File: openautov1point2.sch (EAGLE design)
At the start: 78 parts, among them CN1 6p-2.54, CN2 6p-2.54, CN3 6p-2.54, IC1 NC7SZ14M5X, IC2 TJA1049, IC3 NCP1117CORRECT, J3 4p-2.54, Q1 s9013, Q2 s9013, U3 MMA7660FCR1, U5 A2235-H, U8 PCF85063TP, X3 BU-SMA-H, X4 ABS07-32.768KHZ

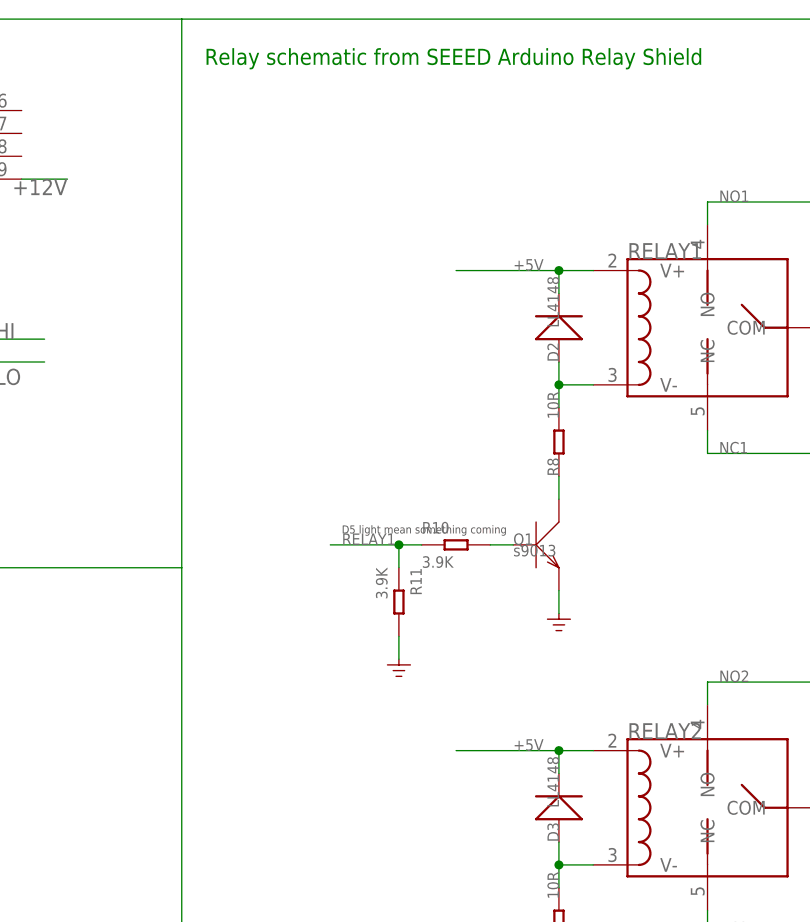
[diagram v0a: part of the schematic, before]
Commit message: updated after design review
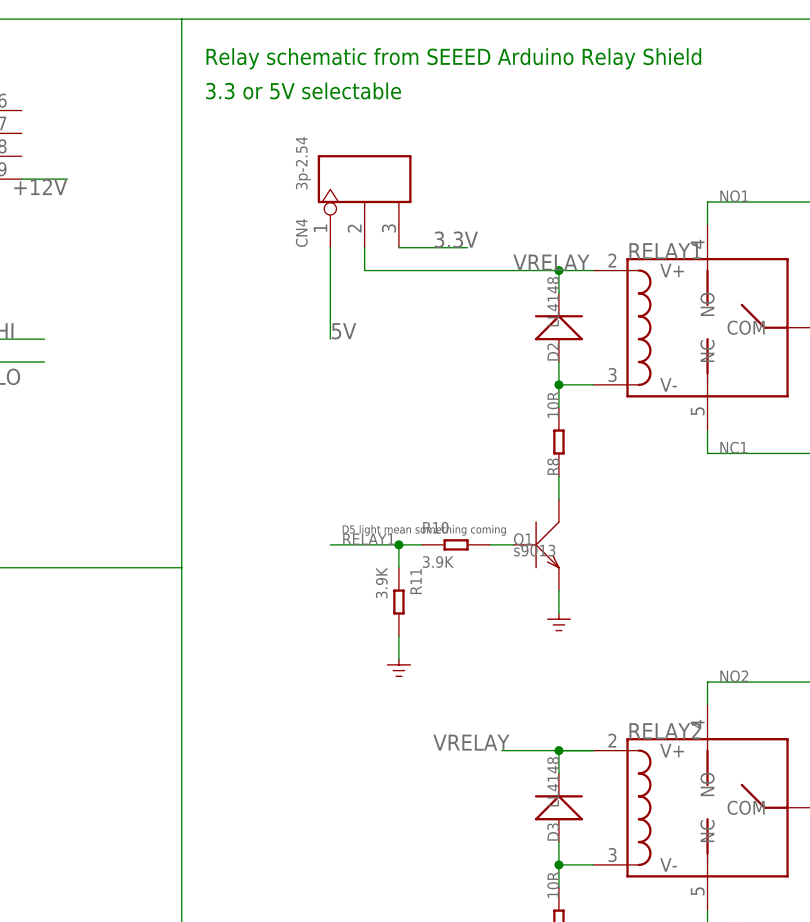
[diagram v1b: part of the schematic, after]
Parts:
- added CN4: 3p-2.54, Seeed-Connector:DIP-BLACK-MALE-HEADER-VERT(3P-2.54)
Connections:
- new net VRELAY: CN4.P$2, D2.-, D3.-, RELAY1.V+, RELAY2.V+
- net +5V: no longer D2.-, D3.-, RELAY1.V+, RELAY2.V+
- net 3.3V: now also CN4.P$3
- net 5V: now also CN4.P$1
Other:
- note added: "3.3 or 5V selectable"
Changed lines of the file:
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@@
 <setting verticaltext="up"/>
 </settings>
-<grid distance="0.1" unitdist="inch" unit="inch" style="lines" multiple="1" display="no" altdistance="0.01" altunitdist="inch" altunit="inch"/>
+<grid distance="0.05" unitdist="inch" unit="inch" style="lines" multiple="1" display="no" altdistance="0.01" altunitdist="inch" altunit="inch"/>
 <layers>
 <layer number="1" name="Top" color="4" fill="1" visible="no" active="no"/>
@@
 <part name="C12" library="Seeed-Capacitor" deviceset="CERAMIC-100NF-50V-10%-X7R(0603)" device="" value="100nf"/>
 <part name="U$12" library="Power or GND " deviceset="GND_POWER" device=""/>
+<part name="CN4" library="Seeed-Connector" deviceset="DIP-BLACK-MALE-HEADER-VERT(3P-2.54)" device="" value="3p-2.54"/>
 </parts>
 <sheets>
@@
 <text x="26.67" y="-54.61" size="1.778" layer="91" rot="R90">Photon</text>
 <text x="26.67" y="-68.58" size="1.778" layer="91" rot="R90">Electron</text>
+<text x="254" y="102.87" size="1.778" layer="91">3.3 or 5V selectable</text>
 </plain>
 <instances>
@@
 </instance>
 <instance part="U$12" gate="G$1" x="412.75" y="-7.62" rot="R90"/>
+<instance part="CN4" gate="G$1" x="271.78" y="93.98" rot="R90"/>
 </instances>
 <busses>
@@
 <net name="+5V" class="2">
 <segment>
-<wire x1="297.18" y1="83.82" x2="293.37" y2="83.82" width="0.1524" layer="91"/>
-<wire x1="293.37" y1="81.28" x2="293.37" y2="83.82" width="0.1524" layer="91"/>
-<wire x1="293.37" y1="83.82" x2="281.94" y2="83.82" width="0.1524" layer="91"/>
-<junction x="293.37" y="83.82"/>
-<label x="288.29" y="83.82" size="1.27" layer="95"/>
-<pinref part="D2" gate="D" pin="-"/>
-<pinref part="RELAY1" gate="G$1" pin="V+"/>
-</segment>
-<segment>
-<wire x1="297.18" y1="30.48" x2="293.37" y2="30.48" width="0.1524" layer="91"/>
-<wire x1="293.37" y1="30.48" x2="281.94" y2="30.48" width="0.1524" layer="91"/>
-<wire x1="293.37" y1="27.94" x2="293.37" y2="30.48" width="0.1524" layer="91"/>
-<junction x="293.37" y="30.48"/>
-<label x="288.29" y="30.48" size="1.27" layer="95"/>
-<pinref part="D3" gate="D" pin="-"/>
-<pinref part="RELAY2" gate="G$1" pin="V+"/>
-</segment>
-<segment>
 <pinref part="CN2" gate="G$1" pin="5"/>
 <wire x1="485.14" y1="85.09" x2="461.01" y2="85.09" width="0.1524" layer="91"/>
@@
 <pinref part="R19" gate="G$1" pin="1"/>
 </segment>
+<segment>
+<pinref part="CN4" gate="G$1" pin="P$3"/>
+<wire x1="275.59" y1="86.36" x2="283.21" y2="86.36" width="0.1524" layer="91"/>
+<label x="279.4" y="86.36" size="1.778" layer="95"/>
+</segment>
 </net>
 <net name="5V" class="1">
@@
 <pinref part="C11" gate="G$1" pin="1"/>
 <wire x1="232.41" y1="-55.88" x2="232.41" y2="-48.26" width="0.1524" layer="91"/>
+</segment>
+<segment>
+<pinref part="CN4" gate="G$1" pin="P$1"/>
+<wire x1="267.97" y1="86.36" x2="267.97" y2="76.2" width="0.1524" layer="91"/>
+<label x="267.97" y="76.2" size="1.778" layer="95"/>
 </segment>
 </net>
@@
 </segment>
 </net>
+<net name="VRELAY" class="0">
+<segment>
+<pinref part="CN4" gate="G$1" pin="P$2"/>
+<wire x1="271.78" y1="86.36" x2="271.78" y2="83.82" width="0.1524" layer="91"/>
+<pinref part="RELAY1" gate="G$1" pin="V+"/>
+<wire x1="271.78" y1="83.82" x2="293.37" y2="83.82" width="0.1524" layer="91"/>
+<pinref part="D2" gate="D" pin="-"/>
+<wire x1="293.37" y1="83.82" x2="297.18" y2="83.82" width="0.1524" layer="91"/>
+<wire x1="293.37" y1="81.28" x2="293.37" y2="83.82" width="0.1524" layer="91"/>
+<junction x="293.37" y="83.82"/>
+<label x="288.29" y="83.82" size="1.778" layer="95"/>
+</segment>
+<segment>
+<pinref part="D3" gate="D" pin="-"/>
+<wire x1="293.37" y1="27.94" x2="293.37" y2="30.48" width="0.1524" layer="91"/>
+<pinref part="RELAY2" gate="G$1" pin="V+"/>
+<wire x1="293.37" y1="30.48" x2="297.18" y2="30.48" width="0.1524" layer="91"/>
+<wire x1="297.18" y1="30.48" x2="293.37" y2="30.48" width="0.1524" layer="91"/>
+<junction x="293.37" y="30.48"/>
+<wire x1="293.37" y1="30.48" x2="287.02" y2="30.48" width="0.1524" layer="91"/>
+<label x="279.4" y="30.48" size="1.778" layer="95"/>
+</segment>
+</net>
